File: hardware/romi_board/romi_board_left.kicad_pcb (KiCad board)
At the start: 2 copper layers, 99.1 x 66 mm, 33 parts, among them J1 Conn_01x14, J2 Conn_01x14, J3 Conn_01x04, SW1 SW_SPST, U1 Teensy4.0

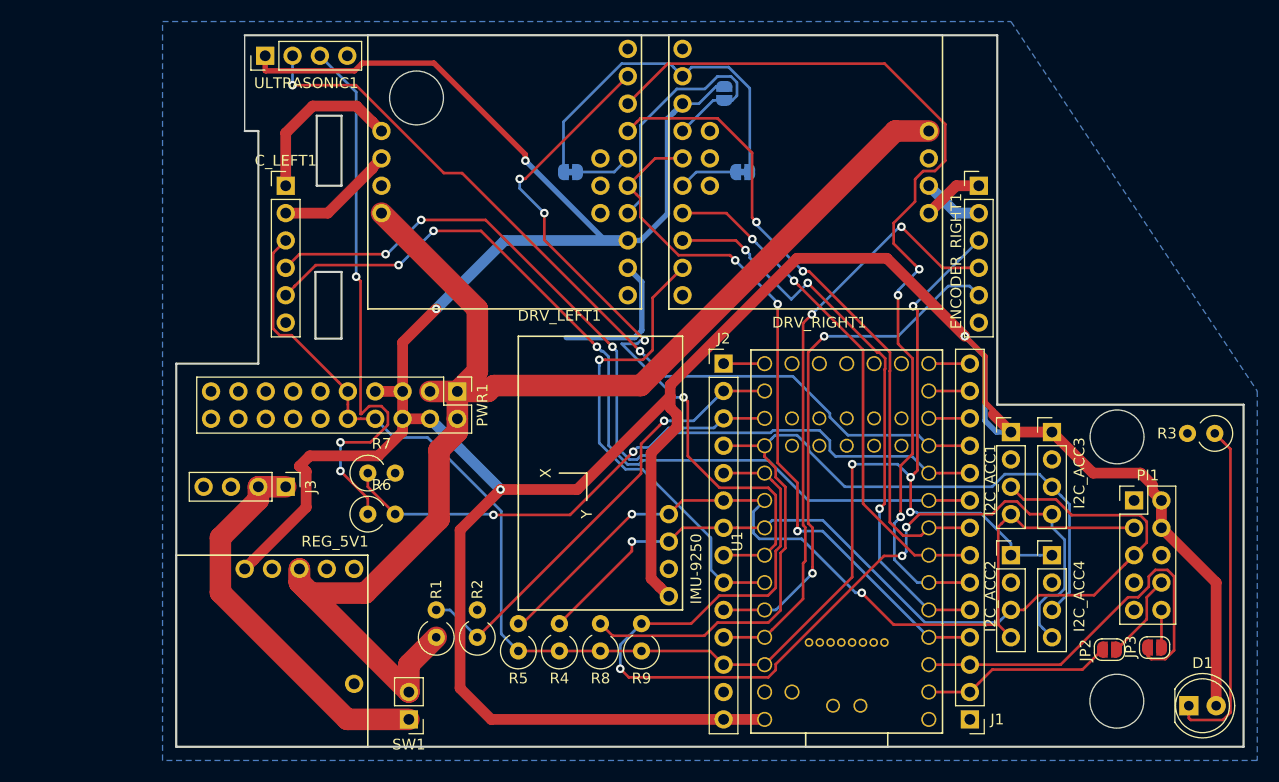
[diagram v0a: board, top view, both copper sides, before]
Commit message: Initial version of schematics and boards.
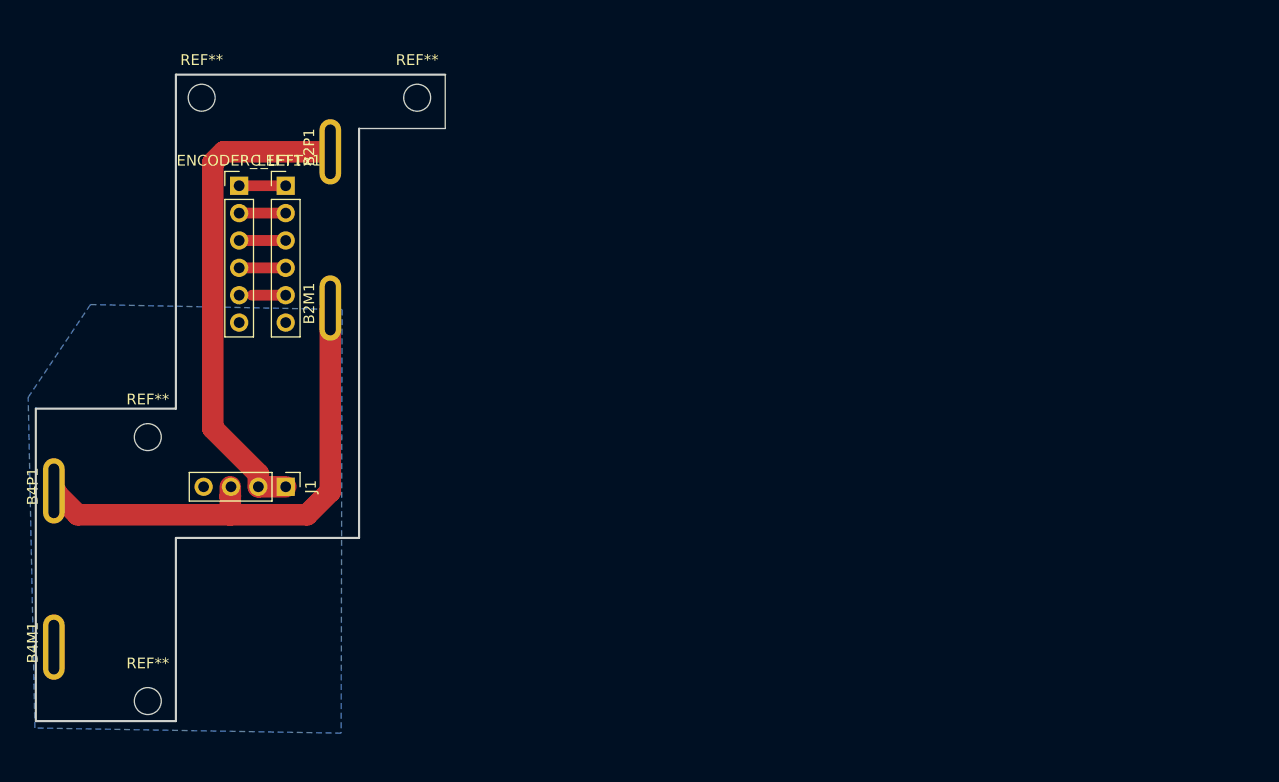
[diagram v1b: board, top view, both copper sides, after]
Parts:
- removed C_LEFT1: Conn_01x07, Connector_PinHeader_2.54mm:PinHeader_1x06_P2.54mm_Vertical
- removed D1: LED, LED_THT:LED_D5.0mm
- removed DRV_LEFT1, DRV_RIGHT1: TB9051FTG, teensy:TB9051FTG_db
- removed ENCODER_RIGHT1: Conn_01x06, Connector_PinHeader_2.54mm:PinHeader_1x06_P2.54mm_Vertical
- removed I2C_ACC1, I2C_ACC2, I2C_ACC3, I2C_ACC4, J3, ULTRASONIC1: Conn_01x04, Connector_PinHeader_2.54mm:PinHeader_1x04_P2.54mm_Vertical
- removed IMU-9250: Conn_01x04, teensy:MPU9250_BB
- removed J2: Conn_01x14, Connector_PinHeader_2.54mm:PinHeader_1x14_P2.54mm_Vertical
- removed JP1, JP2, JP3: SolderJumper_2_Open, Jumper:SolderJumper-2_P1.3mm_Open_RoundedPad1.0x1.5mm
- removed JP4, JP5: SolderJumper_2_Bridged, Jumper:SolderJumper-2_P1.3mm_Bridged_RoundedPad1.0x1.5mm
- removed PI1: RASPBERRY_PI_GPIO, Connector_PinHeader_2.54mm:PinHeader_2x05_P2.54mm_Vertical
- removed PWR1: Conn_02x10_Counter_Clockwise, Connector_PinHeader_2.54mm:PinHeader_2x10_P2.54mm_Vertical
- removed R1, R2, R3, R4, R5, R8, R9: R_US, Resistor_THT:R_Axial_DIN0309_L9.0mm_D3.2mm_P2.54mm_Vertical
- removed R6, R7: R_Small_US, Resistor_THT:R_Axial_DIN0309_L9.0mm_D3.2mm_P2.54mm_Vertical
- removed REG_5V1: D24V22F5, teensy:D24V2F5_bb
- removed SW1: SW_SPST, Connector_PinHeader_2.54mm:PinHeader_1x02_P2.54mm_Vertical
- removed U1: Teensy4.0, teensy:Teensy40_SMT
- added B2M1: BTAB, teensy:romi_battery_tab, F.Cu at (73.3, 112.7)
- added B2P1: BTAB, teensy:romi_battery_tab, F.Cu at (73.3, 98.2)
- added B4M1: BTAB, teensy:romi_battery_tab, F.Cu at (47.7, 144.1)
- added B4P1: BTAB, teensy:romi_battery_tab, F.Cu at (47.7, 129.6)
- added C_LEFTx1: Conn_01x07, Connector_PinHeader_2.54mm:PinHeader_1x06_P2.54mm_Vertical, F.Cu at (69.2, 101.3)
- added ENCODER_LEFT1: Conn_01x06, Connector_PinHeader_2.54mm:PinHeader_1x06_P2.54mm_Vertical, F.Cu at (64.9, 101.3)
- added REF**: MountingHole_2.5mm, MountingHole:MountingHole_2.5mm, F.Cu at (61.4, 93.1)
- added REF**: MountingHole_2.5mm, MountingHole:MountingHole_2.5mm, F.Cu at (56.4, 124.6)
- added REF**: MountingHole_2.5mm, MountingHole:MountingHole_2.5mm, F.Cu at (81.4, 93.1)
- added REF**: MountingHole_2.5mm, MountingHole:MountingHole_2.5mm, F.Cu at (56.4, 149.1)
- J1: value Conn_01x14 -> Conn_01x04; footprint Connector_PinHeader_2.54mm:PinHeader_1x14_P2.54mm_Vertical -> Connector_PinHeader_2.54mm:PinHeader_1x04_P2.54mm_Vertical
- moved J1 67.1 mm to (69.2, 129.3), turned to 270 degrees
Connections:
- J1 pad 1: GND -> +BATT
- J1 pad 2: /TSY_RX -> +BATT
- J1 pad 3: /TSY_TX -> /VBAT_MID
- J1 pad 4: /XD_EN -> GND
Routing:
- net +5V: track 318.9 -> 0.00 mm, vias 4 -> 0
- net +3V3: track 146.9 -> 0.00 mm, vias 4 -> 0
- net +VSW: track 129.1 -> 0.00 mm
- net /I2C2_SDA: track 97.3 -> 0.00 mm, vias 3 -> 0
- net /LD_PWM1: track 87.3 -> 0.00 mm, vias 3 -> 0
- net /LENCA: track 83.1 -> 0.00 mm, vias 3 -> 0
- net /I2C1_SCL: track 81.9 -> 0.00 mm, vias 1 -> 0
- net /I2C1_SDA: track 81.6 -> 0.00 mm, vias 2 -> 0
- net /LENCB: track 81.5 -> 0.00 mm, vias 3 -> 0
- net /I2C2_SCL: track 81.2 -> 0.00 mm
- net /US_TRIG: track 79.7 -> 0.00 mm, vias 2 -> 0
- net /LD_OCM: track 68.9 -> 0.00 mm, vias 4 -> 0
- net /XD_EN: track 67.6 -> 0.00 mm, vias 3 -> 0
- net /LD_PWM2: track 61.5 -> 0.00 mm, vias 2 -> 0
- net /RENCA: track 55.9 -> 0.00 mm, vias 2 -> 0
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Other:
- board size 99.1 x 66 mm -> 38 x 60 mm
- net class Motor removed
- net class PWR added: clearance 0.6, trace_width 2, via_dia 0.8, via_drill 0.4
- net class Supply removed
